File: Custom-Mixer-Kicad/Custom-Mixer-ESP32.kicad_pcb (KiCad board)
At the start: 2 copper layers, 162.2 x 127.6 mm, 38 parts, among them J1 Conn_01x08, SW1 RotaryEncoder_Switch, SW10 SW_Push, SW11 SW_Push, SW12 SW_Push, SW13 SW_Push, SW14 SW_Push, SW15 SW_Push, SW16 SW_Push, SW17 SW_Push, SW18 SW_Push, SW2 RotaryEncoder_Switch, SW21 SW_Push, SW3 SW_Push, SW4 SW_Push, SW5 SW_Push, SW6 SW_Push, SW7 SW_Push, SW8 SW_Push, SW9 SW_Push, U7 ESP32-S3-DevKitC, U8 MCP23017_SP

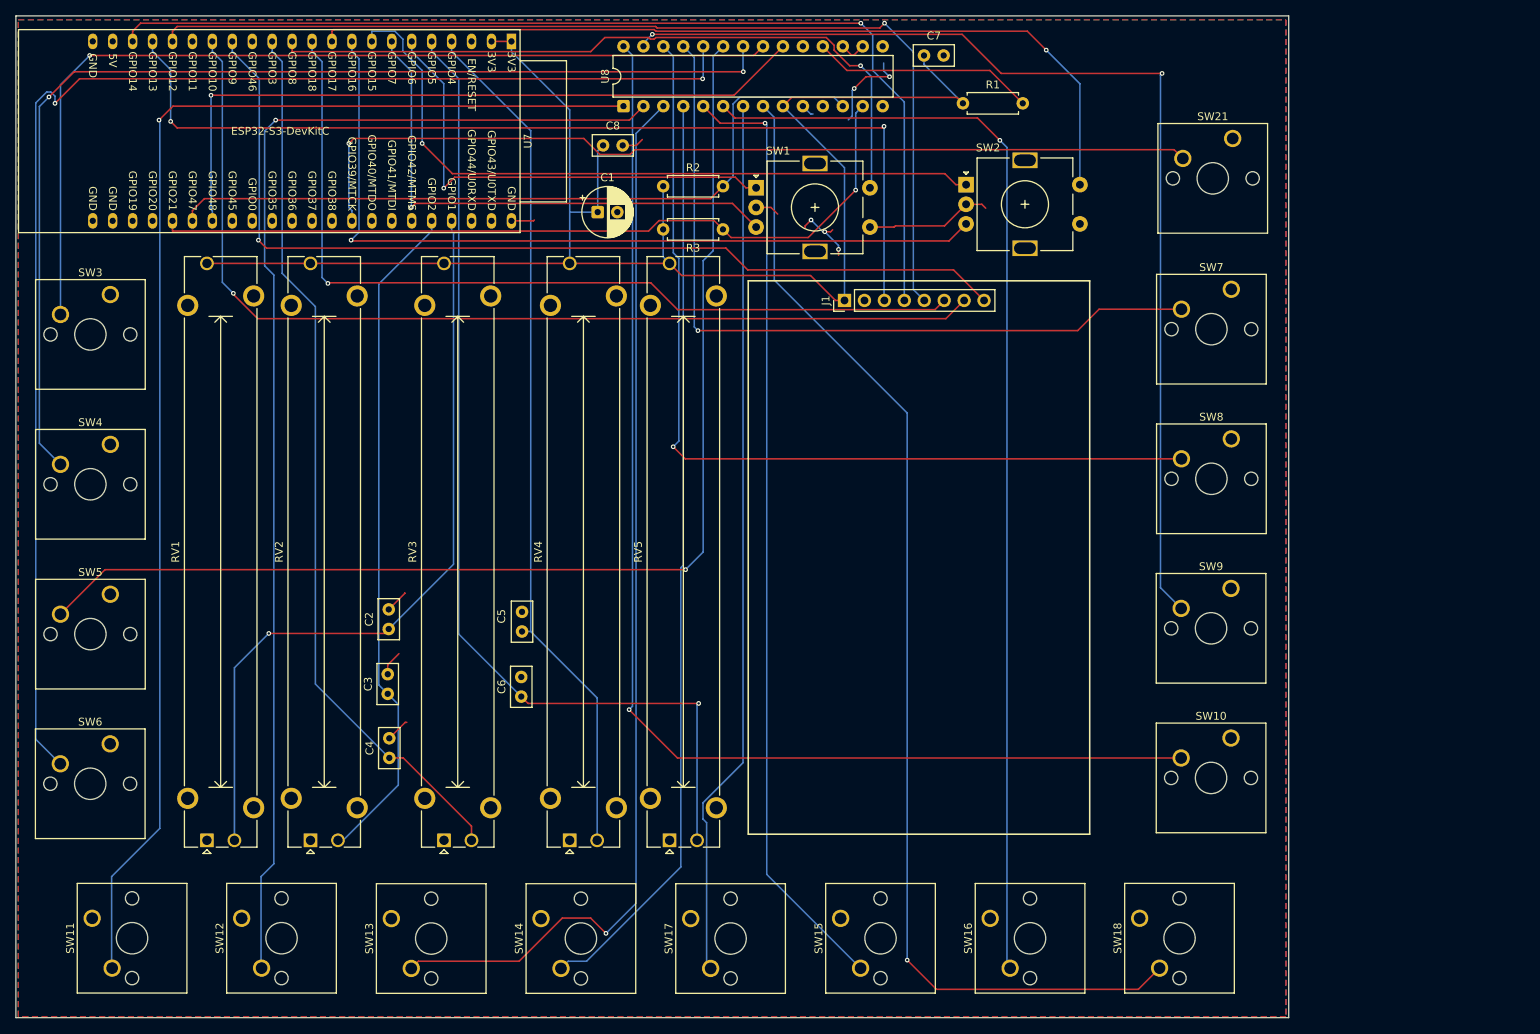
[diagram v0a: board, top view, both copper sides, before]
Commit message: Update Custom-Mixer-ESP32.kicad_pcb
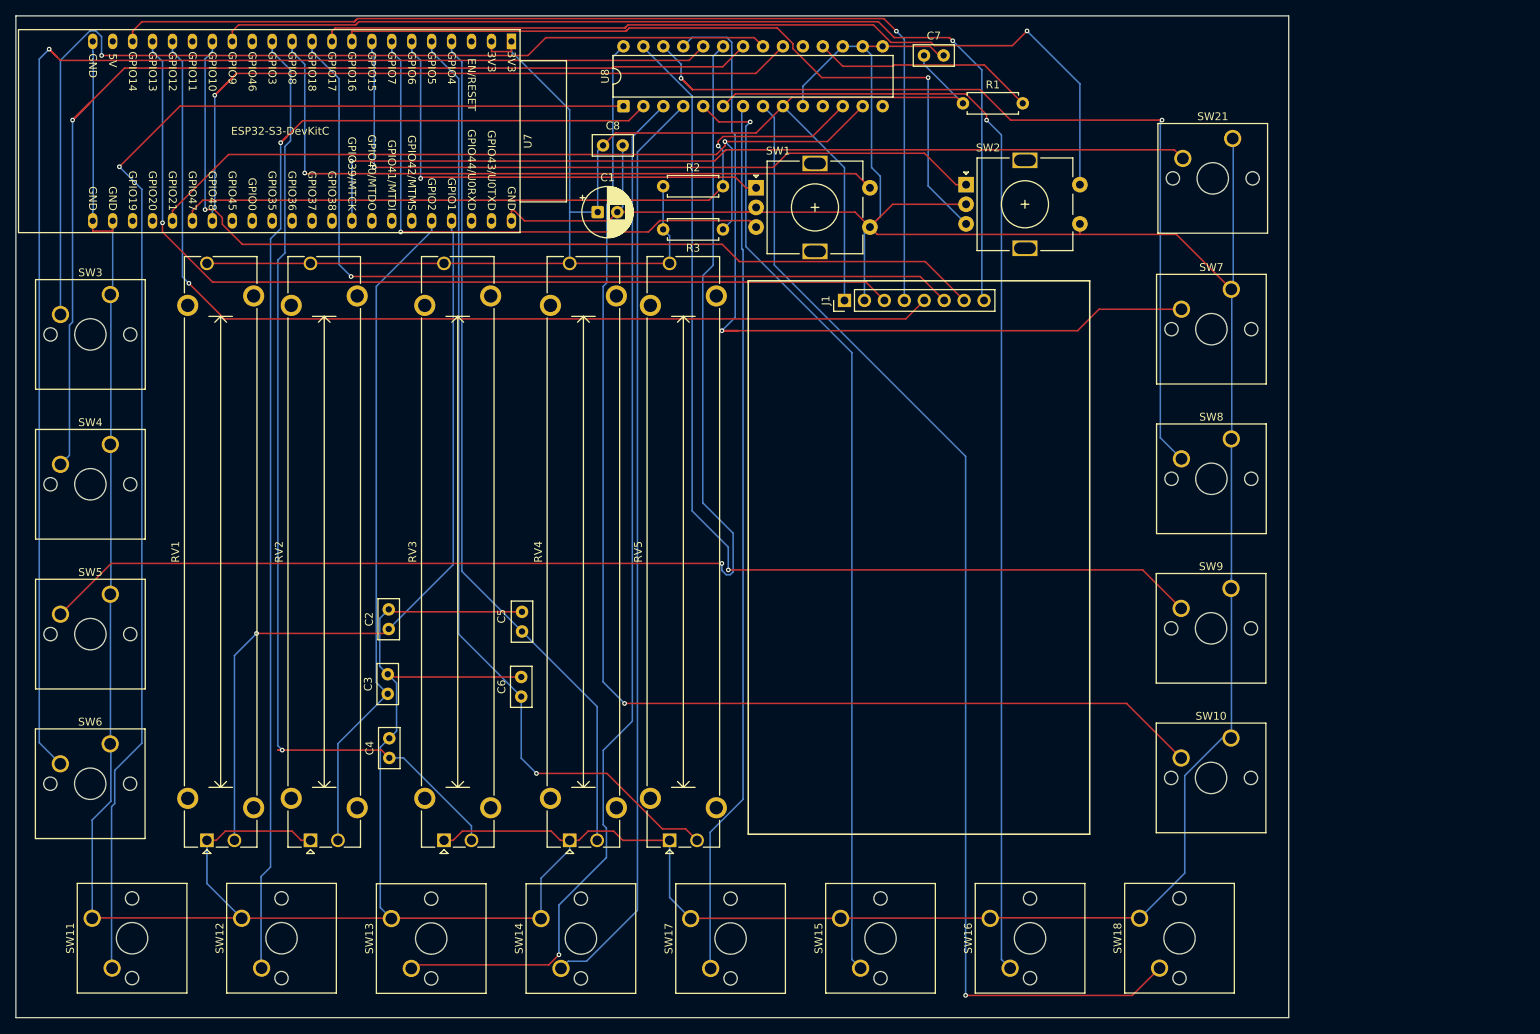
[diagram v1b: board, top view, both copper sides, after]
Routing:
- net GND: track 59.4 -> 675.1 mm, vias 5 -> 0
- net Net-(U7-GPIO48): track 91.5 -> 106.8 mm
- net a4: track 99.7 -> 112.6 mm
- net GPIO 3: track 113.3 -> 124.3 mm, vias 0 -> 1
- net a2: track 150.6 -> 159.3 mm
- net a6: track 138.3 -> 130.9 mm, vias 2 -> 1
- net BL: track 122.4 -> 129.6 mm
- net a0: track 120.8 -> 127.5 mm
- net GPIO 16: track 105.4 -> 98.7 mm
- net GPIO 5: track 128.7 -> 122.8 mm
- net a3: track 177.6 -> 183.0 mm, vias 2 -> 1
- net a1: track 141.5 -> 146.4 mm, vias 2 -> 1
- net RST: track 128.7 -> 123.8 mm
- net a5: track 117.5 -> 122.3 mm, vias 1 -> 2
- net MOSI: track 124.7 -> 120.4 mm, vias 2 -> 1
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- removed copper zone on B.Cu, net GND
- removed copper zone on F.Cu, net GND

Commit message: Complete Wire Revamp
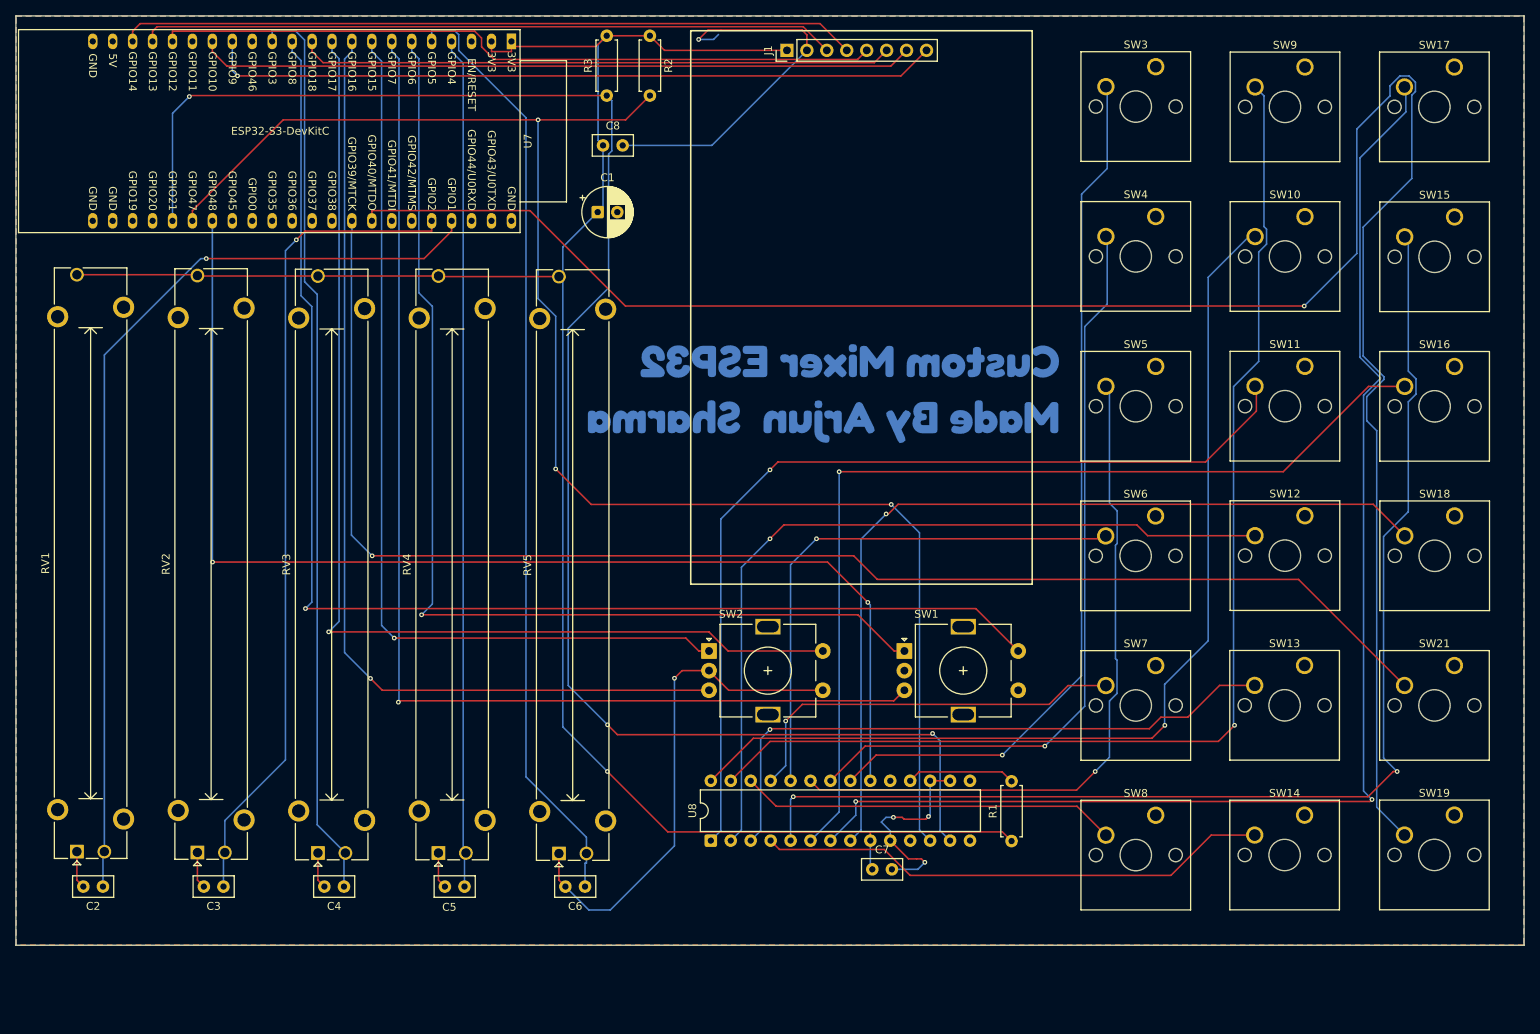
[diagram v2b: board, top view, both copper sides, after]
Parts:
- added SW19: SW_Push, Button_Switch_Keyboard:SW_Cherry_MX_1.00u_PCB, F.Cu at (281.4, 160.8)
- added kibuzzard-6987AAB7: G***, kibuzzard-6987AAB7, B.Cu at (201.1, 107.1)
- moved SW11 169.7 mm to (262.4, 103.6), turned to 0 degrees
- moved SW17 145.7 mm to (281.4, 65.5), turned to 0 degrees
- moved SW12 144.8 mm to (262.4, 122.7), turned to 0 degrees
- moved SW3 136.3 mm to (243.4, 65.5)
- moved SW4 136.3 mm to (243.4, 84.6)
- moved SW5 136.3 mm to (243.4, 103.7)
- moved SW6 136.3 mm to (243.4, 122.7)
- moved SW13 120.7 mm to (262.4, 141.8), turned to 0 degrees
- moved SW15 118.8 mm to (281.5, 84.6), turned to 0 degrees
- moved C7 103.9 mm to (207.3, 167.7)
- moved SW14 98.2 mm to (262.4, 160.8), turned to 0 degrees
- moved U8 94.2 mm to (186.7, 164.1)
- moved R1 94.2 mm to (225.0, 164.1), turned to 90 degrees
- moved SW16 91.9 mm to (281.5, 103.7), turned to 0 degrees
- moved SW21 72.8 mm to (281.5, 141.8)
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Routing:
- net GND: track 675.1 -> 157.9 mm, vias 0 -> 5
- net GPIO 40: track 0.00 -> 264.4 mm, vias 0 -> 1
- net a3: track 183.0 -> 69.2 mm
- net SCL: track 93.9 -> 200.6 mm, vias 1 -> 3
- net SDA: track 107.1 -> 211.3 mm, vias 1 -> 3
- net GPIO 7: track 71.0 -> 149.7 mm
- net GPIO 6: track 61.3 -> 138.1 mm
- net GPIO 8: track 90.2 -> 166.7 mm
- net a5: track 122.3 -> 48.1 mm, vias 2 -> 0
- net a2: track 159.3 -> 88.7 mm
- net GPIO 39: track 114.9 -> 182.2 mm
- net a4: track 112.6 -> 51.1 mm
- net +3V3: track 202.8 -> 262.5 mm, vias 0 -> 1
- net b6: track 112.0 -> 167.9 mm, vias 0 -> 2
- net b1: track 159.1 -> 103.6 mm
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- added copper zone on B.Cu, net GND
- added copper zone on F.Cu, net GND
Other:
- board size 162.2 x 127.6 mm -> 192.1 x 118.4 mm
